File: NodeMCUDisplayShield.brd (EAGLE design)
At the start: 34.3 x 6.7 mm, 2 parts

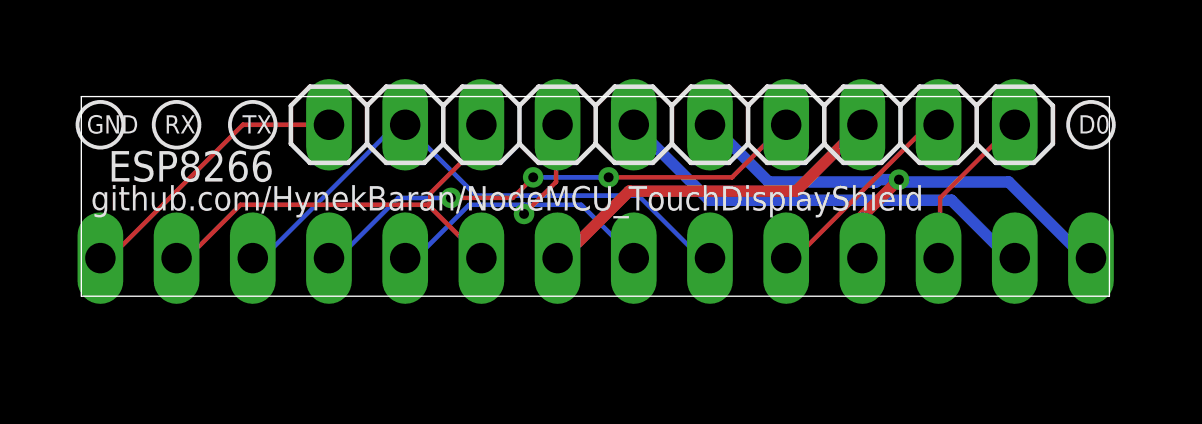
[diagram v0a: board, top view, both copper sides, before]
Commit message: Single-sided version
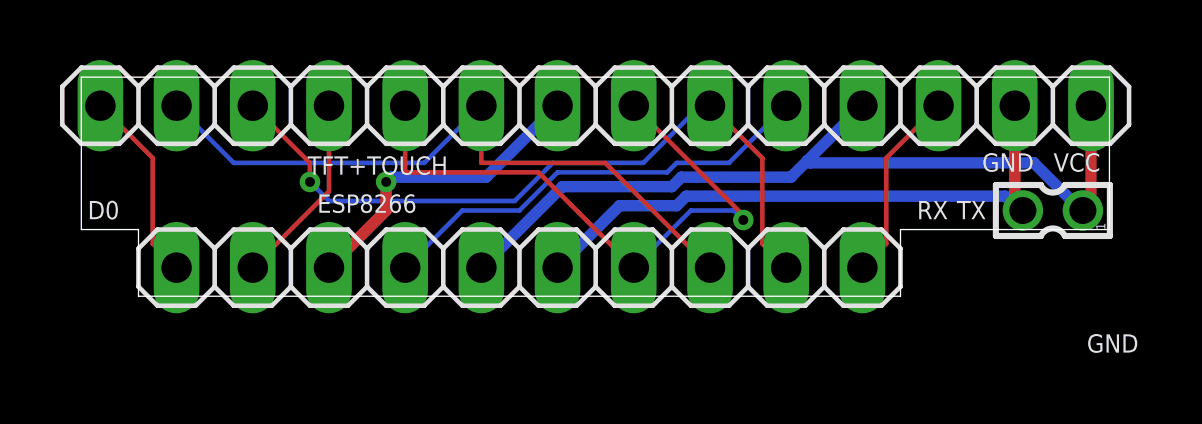
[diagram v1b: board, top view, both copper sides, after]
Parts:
- added X1: 332-02, con-garry:332-02
- moved ESP8266 6.96 mm to (15.2, 0.95), turned to 0 degrees
- moved TFT+TOUCH 5.08 mm to (17.8, 6.35), flipped to the top, turned to 0 degrees
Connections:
- net LED renamed D3
- net SCK renamed D5_SCK
- net SDI/MOSI renamed D7_SDI/MOSI
- net SODI/MISO renamed D6_SODI/MISO
- removed net CS: ESP8266.1, TFT+TOUCH.12
- removed net D/C: ESP8266.2, TFT+TOUCH.10
- removed net T_CS: ESP8266.4, TFT+TOUCH.4
- removed net T_IRQ: ESP8266.10, TFT+TOUCH.1
- new net D1: ESP8266.1, TFT+TOUCH.1
- new net D2: ESP8266.2, TFT+TOUCH.4
- new net D4: ESP8266.4, TFT+TOUCH.10
- new net D8: ESP8266.10, TFT+TOUCH.12
- net GND: now also X1.2
- net VCC: now also X1.1
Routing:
- net T_CS: track 17.1 -> 0.00 mm, vias 3 -> 0
- net D4: track 0.00 -> 14.9 mm
- net VCC: track 17.7 -> 28.5 mm, vias 1 -> 0
- net T_IRQ: track 9.46 -> 0.00 mm
- net D5_SCK: track 12.9 -> 21.1 mm
- net D6_SODI/MISO: track 15.1 -> 22.7 mm
- net D/C: track 6.92 -> 0.00 mm
- net D2: track 0.00 -> 6.45 mm
- net D1: track 0.00 -> 6.45 mm
- net D8: track 0.00 -> 6.45 mm
- net GND: track 14.5 -> 20.4 mm
- net D7_SDI/MOSI: track 18.9 -> 24.7 mm, vias 0 -> 1
- net CS: track 5.54 -> 0.00 mm
- net D3: track 12.0 -> 10.4 mm, vias 0 -> 1
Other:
- board size 34.3 x 6.7 mm -> 34.3 x 7.3 mm
- board text removed: "TOUCH"
